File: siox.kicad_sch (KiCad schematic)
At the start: 1 part, among them U1 MSP430G2131IN14

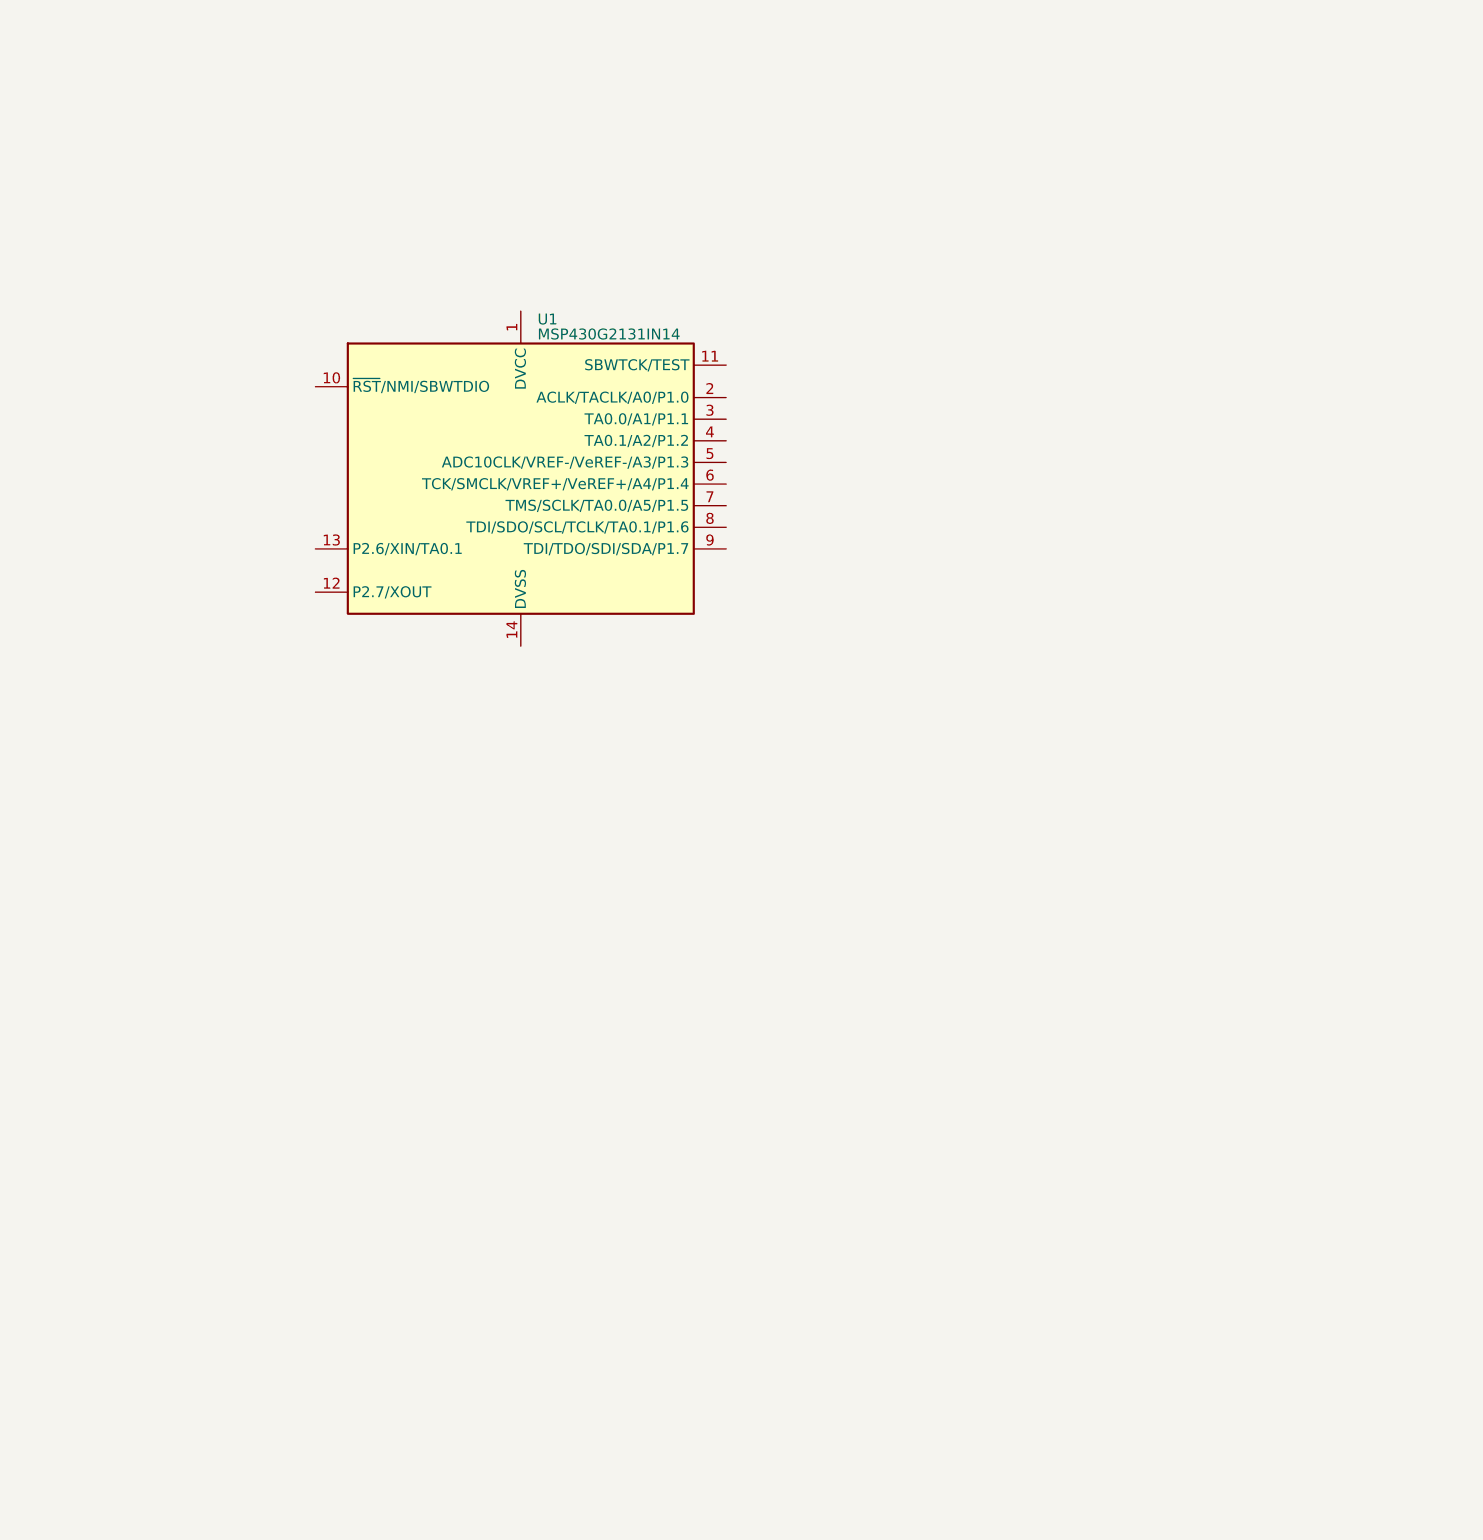
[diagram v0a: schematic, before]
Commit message: fixes
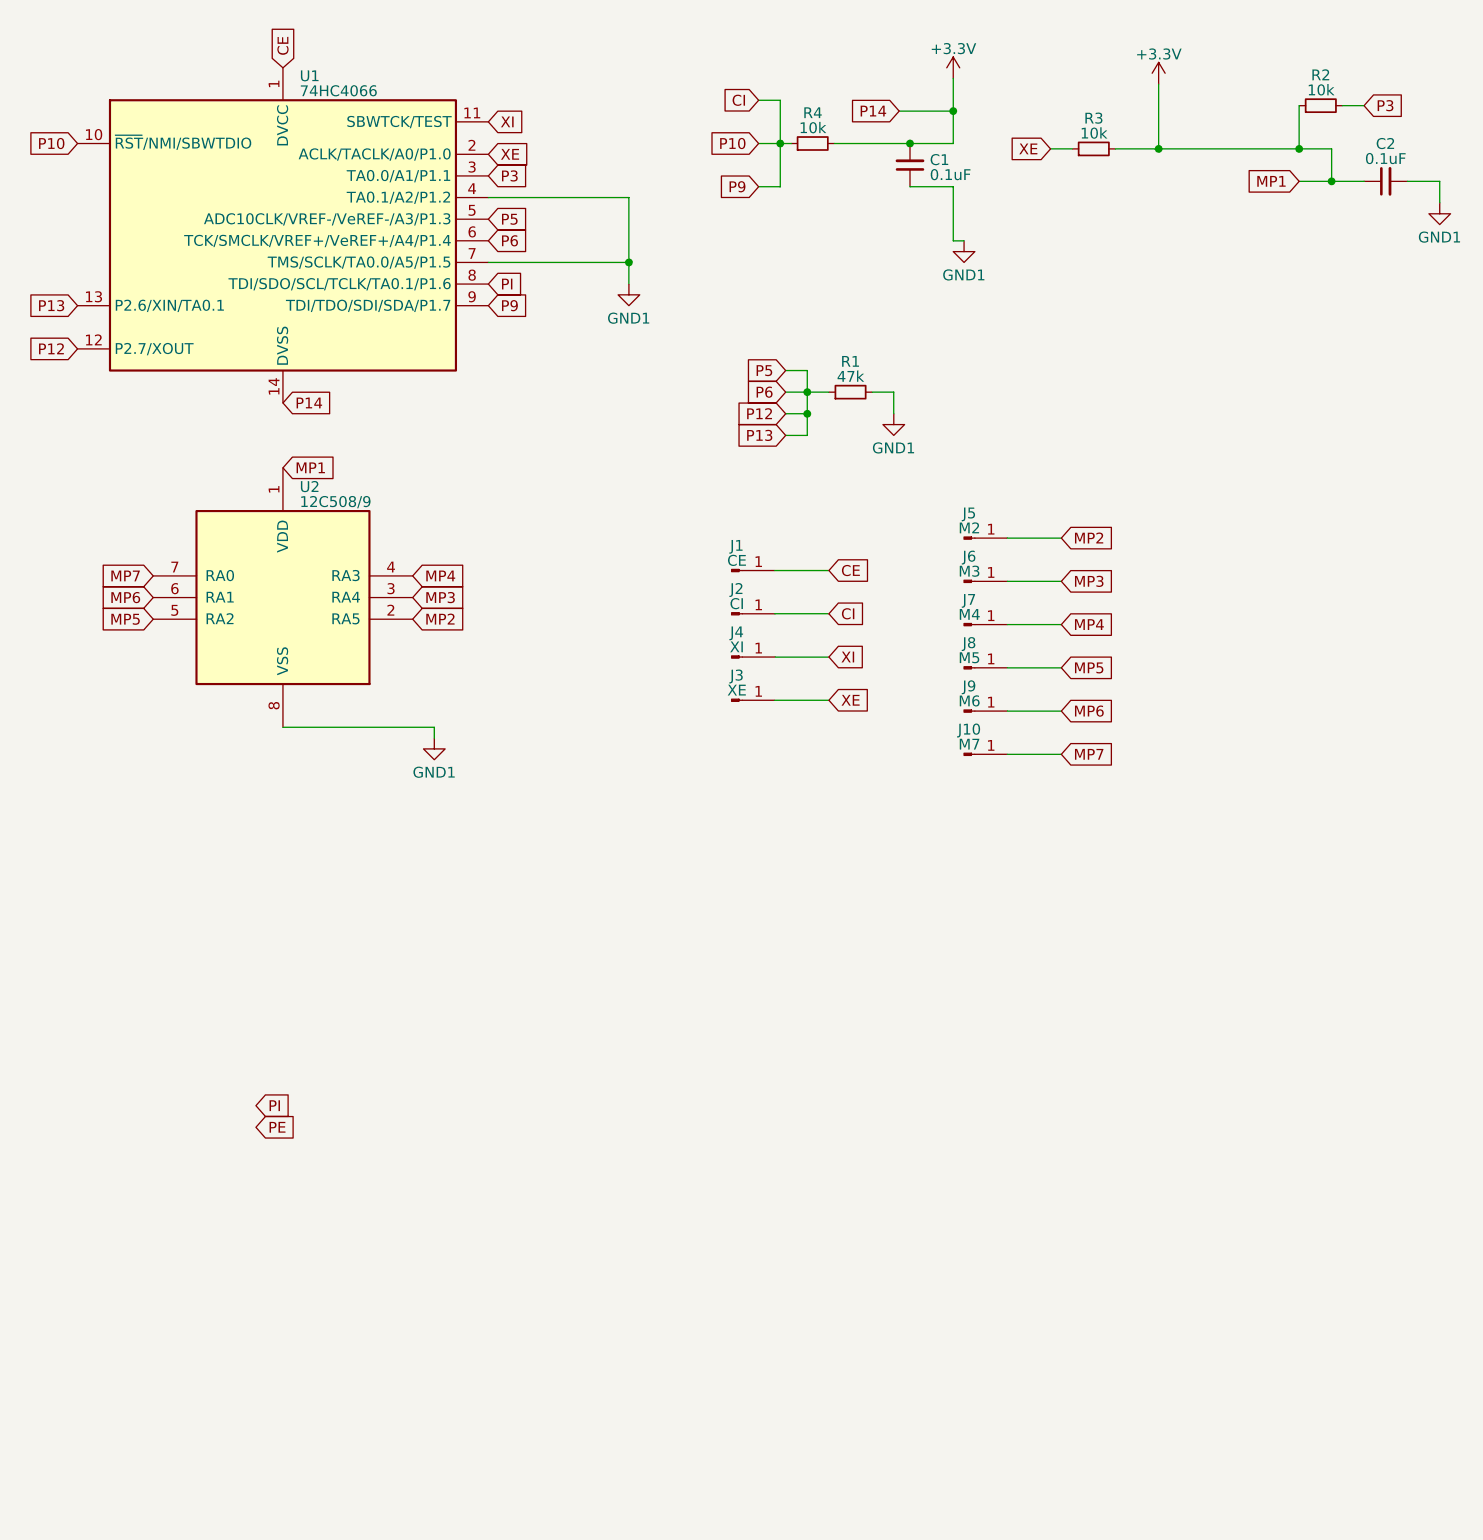
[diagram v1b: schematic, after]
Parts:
- added C1, C2: 0.1uF, Capacitor_SMD:C_0805_2012Metric, symbol Device:C_Small
- added J1: CE, TestPoint:TestPoint_Pad_D2.0mm, symbol Connector:Conn_01x01_Male
- added J10: M7, TestPoint:TestPoint_Pad_D2.0mm, symbol Connector:Conn_01x01_Male
- added J2: CI, TestPoint:TestPoint_Pad_D2.0mm, symbol Connector:Conn_01x01_Male
- added J3: XE, TestPoint:TestPoint_Pad_D2.0mm, symbol Connector:Conn_01x01_Male
- added J4: XI, TestPoint:TestPoint_Pad_D2.0mm, symbol Connector:Conn_01x01_Male
- added J5: M2, TestPoint:TestPoint_Pad_D2.0mm, symbol Connector:Conn_01x01_Male
- added J6: M3, TestPoint:TestPoint_Pad_D2.0mm, symbol Connector:Conn_01x01_Male
- added J7: M4, TestPoint:TestPoint_Pad_D2.0mm, symbol Connector:Conn_01x01_Male
- added J8: M5, TestPoint:TestPoint_Pad_D2.0mm, symbol Connector:Conn_01x01_Male
- added J9: M6, TestPoint:TestPoint_Pad_D2.0mm, symbol Connector:Conn_01x01_Male
- added R1: 47k, Resistor_SMD:R_0805_2012Metric, symbol Device:R_Small
- added R2, R3, R4: 10k, Resistor_SMD:R_0805_2012Metric, symbol Device:R_Small
- added U2: 12C508/9, Package_SO:SOP-8_5.28x5.23mm_P1.27mm, symbol MCU_Microchip_PIC12:PIC12F1501-IMS
- U1: value MSP430G2131IN14 -> 74HC4066
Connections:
- net CE: now reaches U1.1 (DVCC)
- net CE: now also J1.1 (Pin_1)
- net CI: now reaches U1.10 (~{RST}/NMI/SBWTDIO)
- net CI: now also U1.9 (TDI/TDO/SDI/SDA/P1.7), J2.1 (Pin_1), R4.1
- net XI: now reaches U1.11 (SBWTCK/TEST)
- net XI: now also J4.1 (Pin_1)
- net P12: now reaches U1.12 (P2.7/XOUT)
- net P12: now also U1.13 (P2.6/XIN/TA0.1), U1.5 (ADC10CLK/VREF-/VeREF-/A3/P1.3), U1.6 (TCK/SMCLK/VREF+/VeREF+/A4/P1.4), R1.1
- net +3.3V: now reaches U1.14 (DVSS)
- net +3.3V: now also C1.2, C2.1, R2.1, R3.2, R4.2, U2.1 (VDD)
- net XE: now reaches U1.2 (ACLK/TACLK/A0/P1.0)
- net XE: now also J3.1 (Pin_1), R3.1
- net P3: now reaches U1.3 (TA0.0/A1/P1.1)
- net P3: now also R2.2
- net GND1: now reaches U1.4 (TA0.1/A2/P1.2)
- net GND1: now also U1.7 (TMS/SCLK/TA0.0/A5/P1.5), C1.1, C2.2, R1.2, U2.8 (VSS)
- net PI: now reaches U1.8 (TDI/SDO/SCL/TCLK/TA0.1/P1.6)
- new net MP2: J5.1 (Pin_1), U2.2 (RA5)
- new net MP3: J6.1 (Pin_1), U2.3 (RA4)
- new net MP4: J7.1 (Pin_1), U2.4 (RA3)
- new net MP5: J8.1 (Pin_1), U2.5 (RA2)
- new net MP6: J9.1 (Pin_1), U2.6 (RA1)
- new net MP7: J10.1 (Pin_1), U2.7 (RA0)
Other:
- moved on the sheet: U1

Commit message: fix pads
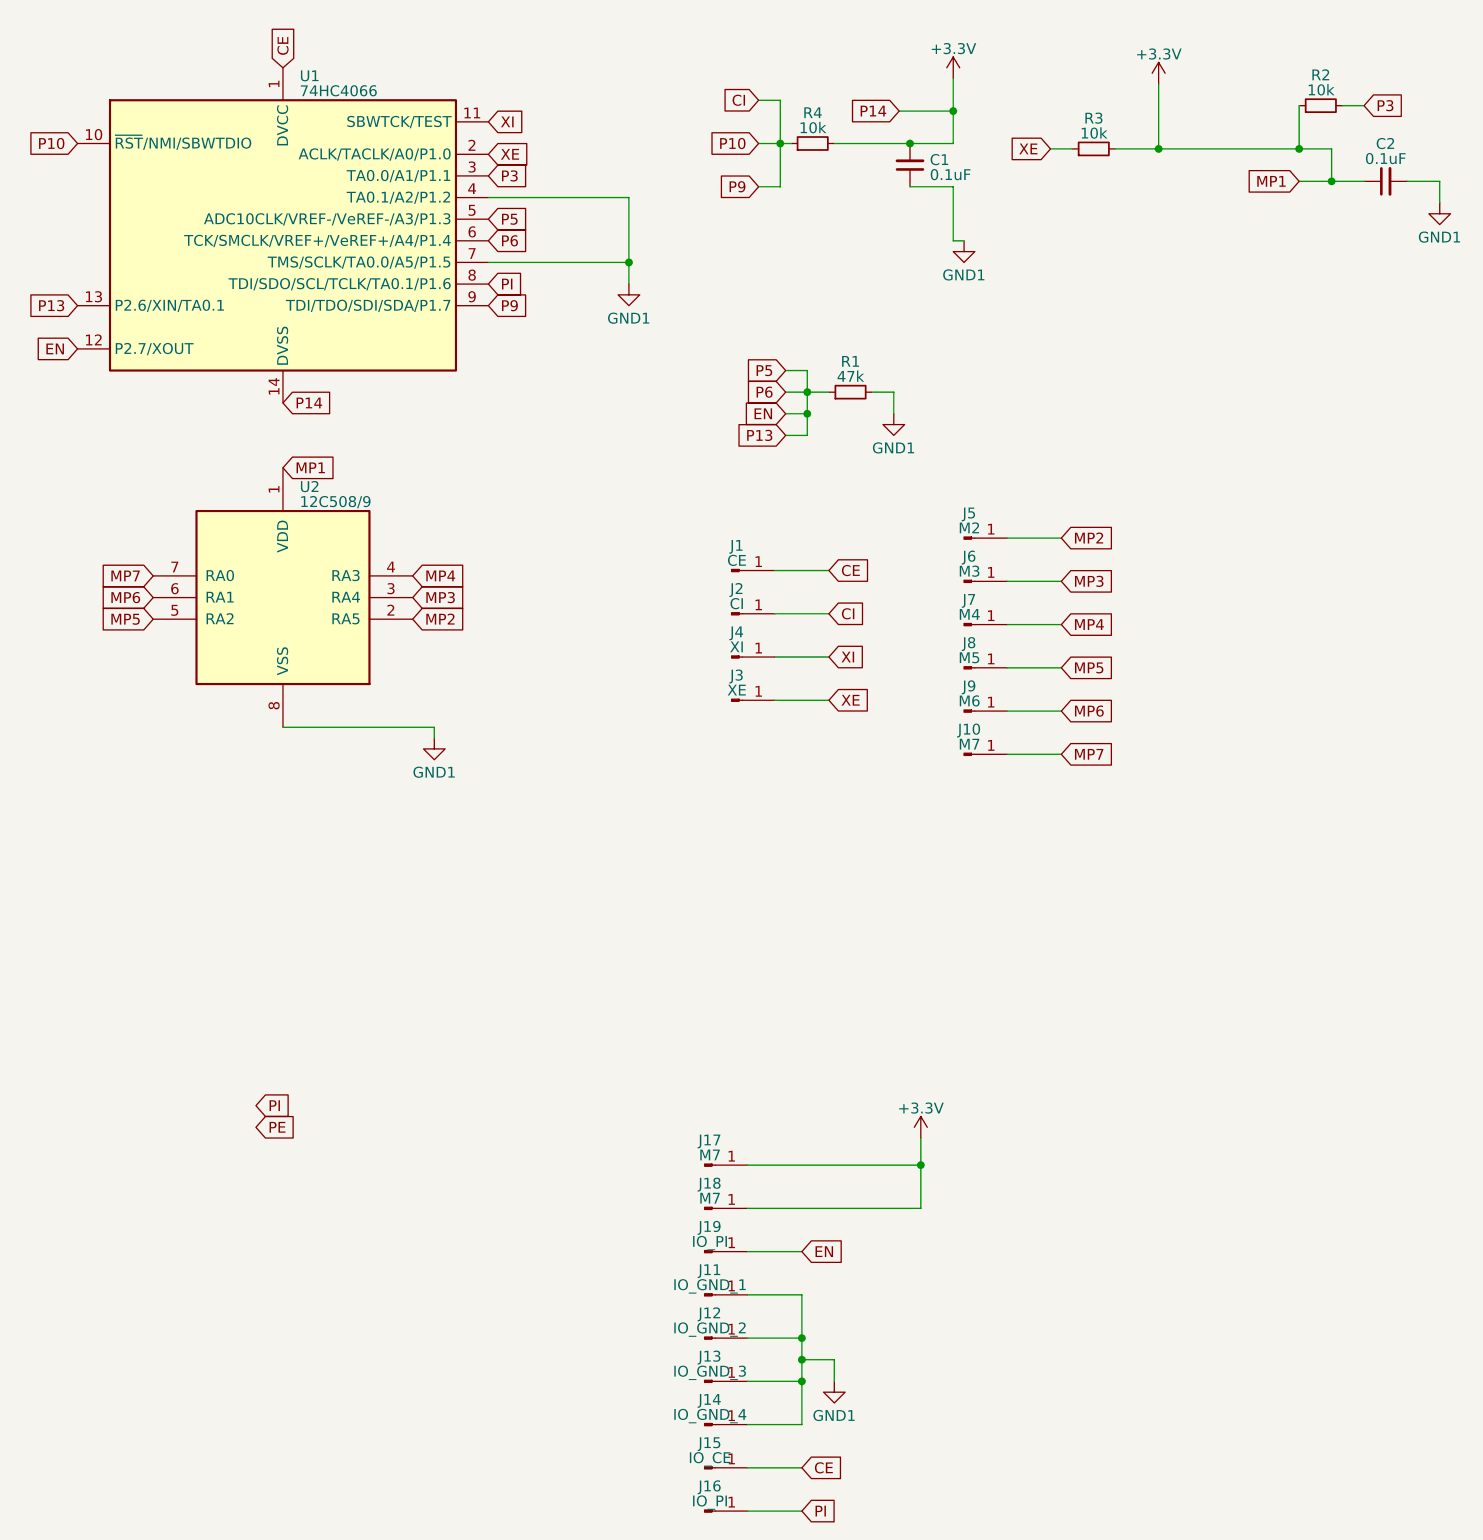
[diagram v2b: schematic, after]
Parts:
- added J11: IO_GND_1, PsioPin:PsioPin, symbol Connector:Conn_01x01_Male
- added J12: IO_GND_2, PsioPin:PsioPin, symbol Connector:Conn_01x01_Male
- added J13: IO_GND_3, PsioPin:PsioPin, symbol Connector:Conn_01x01_Male
- added J14: IO_GND_4, PsioPin:PsioPin, symbol Connector:Conn_01x01_Male
- added J15: IO_CE, PsioPin:PsioPin, symbol Connector:Conn_01x01_Male
- added J16, J19: IO_PI, PsioPin:PsioPin, symbol Connector:Conn_01x01_Male
- added J17, J18: M7, PsioPin:PsioPin, symbol Connector:Conn_01x01_Male
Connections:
- net +3.3V: now also J17.1 (Pin_1), J18.1 (Pin_1)
- net CE: now also J15.1 (Pin_1)
- net GND1: now also J11.1 (Pin_1), J12.1 (Pin_1), J13.1 (Pin_1), J14.1 (Pin_1)
- net PI: now also J16.1 (Pin_1)
- net P12 renamed EN
- net EN: now also J19.1 (Pin_1)
